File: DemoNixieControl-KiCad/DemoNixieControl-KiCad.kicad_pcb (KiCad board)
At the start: 2 copper layers, 110.5 x 71.1 mm, 118 parts, among them J1 TP, J10 TP, J100 TP, J101 TP, J102 TP, J103 Screw_Terminal, J104 Screw_Terminal, J105 Screw_Terminal, J106 Screw_Terminal, J11 TP, J12 TP, J13 TP, J14 TP, J15 TP, J16 TP, J17 TP, J18 TP, J19 TP, J2 TP, J20 TP, J21 TP, J22 TP, J23 TP, J24 TP, J25 TP, J26 TP, J27 TP, J28 TP, J29 TP, J3 TP, J30 TP, J31 TP, J32 TP, J33 TP, J34 TP, J35 HE10_02x10, J36 WAGO256, J37 TP, J38 TP, J39 TP, J4 TP, J40 TP, J41 TP, J42 TP, J43 TP, J44 TP, J45 TP, J46 TP, J47 TP, J48 TP, J49 TP, J5 TP, J50 TP, J51 TP, J52 TP, J53 TP, J54 TP, J55 TP, J56 TP, J57 TP, J58 TP, J59 TP, J6 TP, J60 TP, J61 TP, J62 TP, J63 TP, J64 TP, J65 TP, J66 TP, J67 TP, J68 TP, J69 TP, J7 TP, J70 TP, J71 TP, J72 TP, J73 TP, J74 TP, J75 TP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

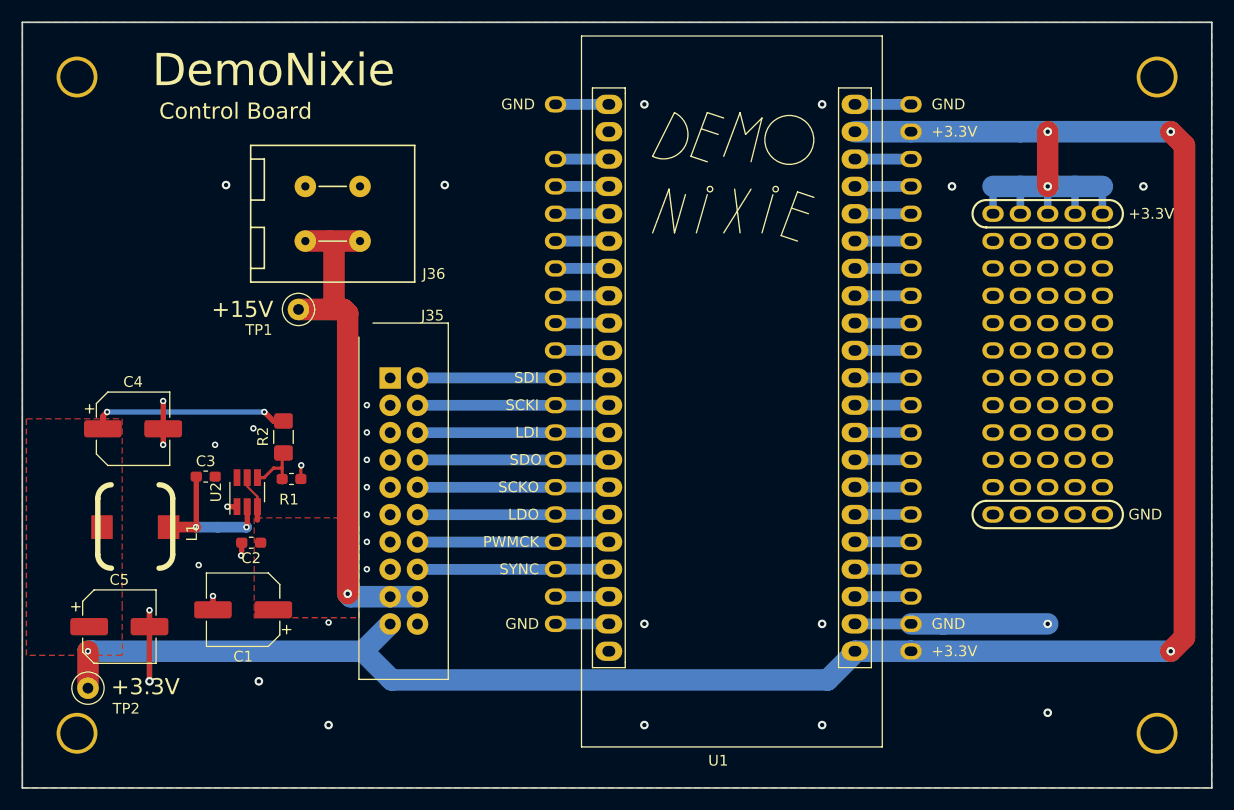
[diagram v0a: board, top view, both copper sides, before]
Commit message: finalisation controlBoard
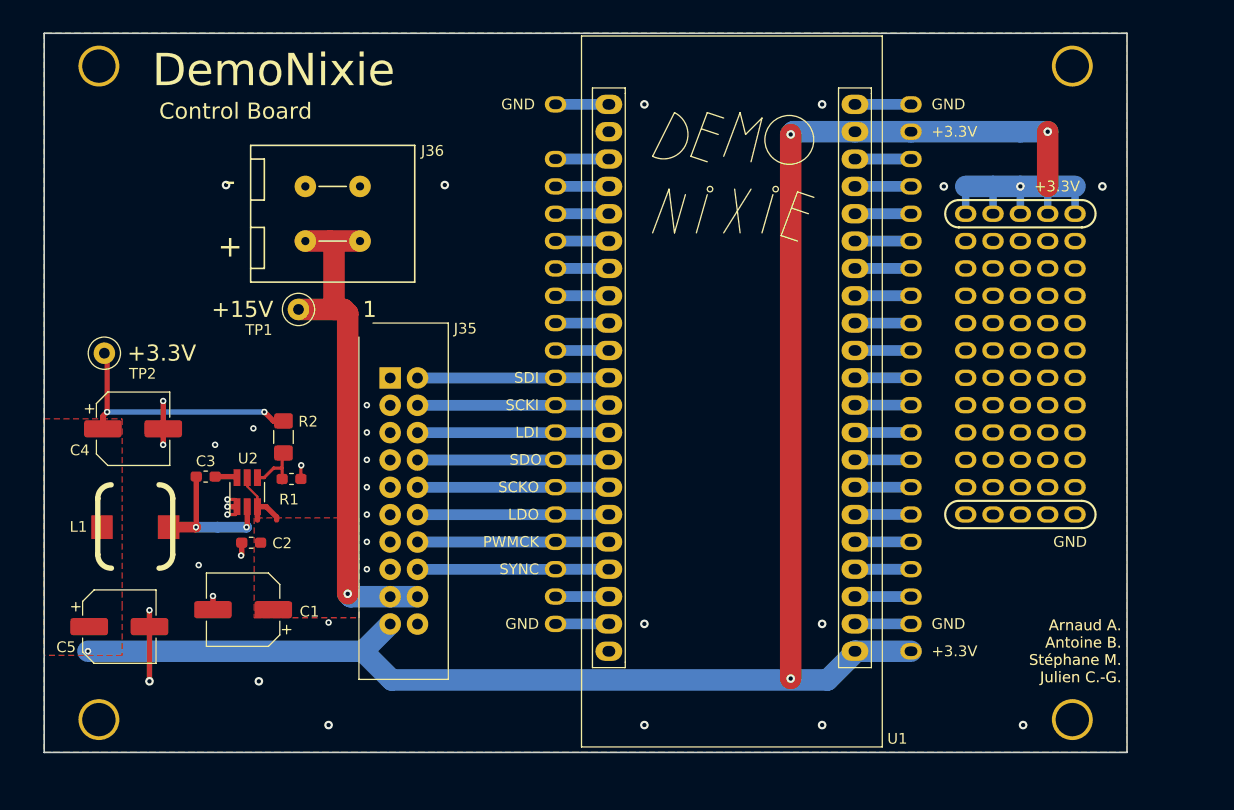
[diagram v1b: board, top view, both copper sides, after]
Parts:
- moved TP2 31.2 mm to (149.5, 94.5)
- moved J106 7.98 mm to (239.4, 128.5)
- moved J104 7.94 mm to (239.4, 67.8)
- moved J102 2.54 mm to (239.6, 109.5)
- moved J38 2.54 mm to (229.5, 86.6)
- moved J40 2.54 mm to (239.6, 84.1)
- moved J44 2.54 mm to (229.5, 99.3)
- moved J45 2.54 mm to (229.5, 84.1)
- moved J46 2.54 mm to (239.6, 91.7)
- moved J48 2.54 mm to (239.6, 89.1)
- moved J51 2.54 mm to (229.5, 94.2)
- moved J56 2.54 mm to (229.5, 89.1)
- moved J59 2.54 mm to (239.6, 94.2)
- moved J61 2.54 mm to (229.5, 91.7)
- moved J62 2.54 mm to (239.6, 86.6)
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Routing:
- net +3V3: track 234.9 -> 208.8 mm
- net GND: track 48.3 -> 38.0 mm, vias 33 -> 34
- net +15V: track 54.2 -> 56.6 mm
- net Net-(C3-Pad2): track 0.00 -> 2.07 mm
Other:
- board size 110.5 x 71.1 mm -> 100.6 x 66.8 mm
- board text added: "+"
- board text added: "-"
- board text added: "1"
- board text added: "Arnaud A. Antoine B. Stéphane M. Julien C.-G."
